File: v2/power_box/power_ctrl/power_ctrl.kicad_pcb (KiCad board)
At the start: 2 copper layers, 37 parts, among them J1 Atmega328, Q1 BC547, Q2 Q_PMOS_GDS, U1 7805

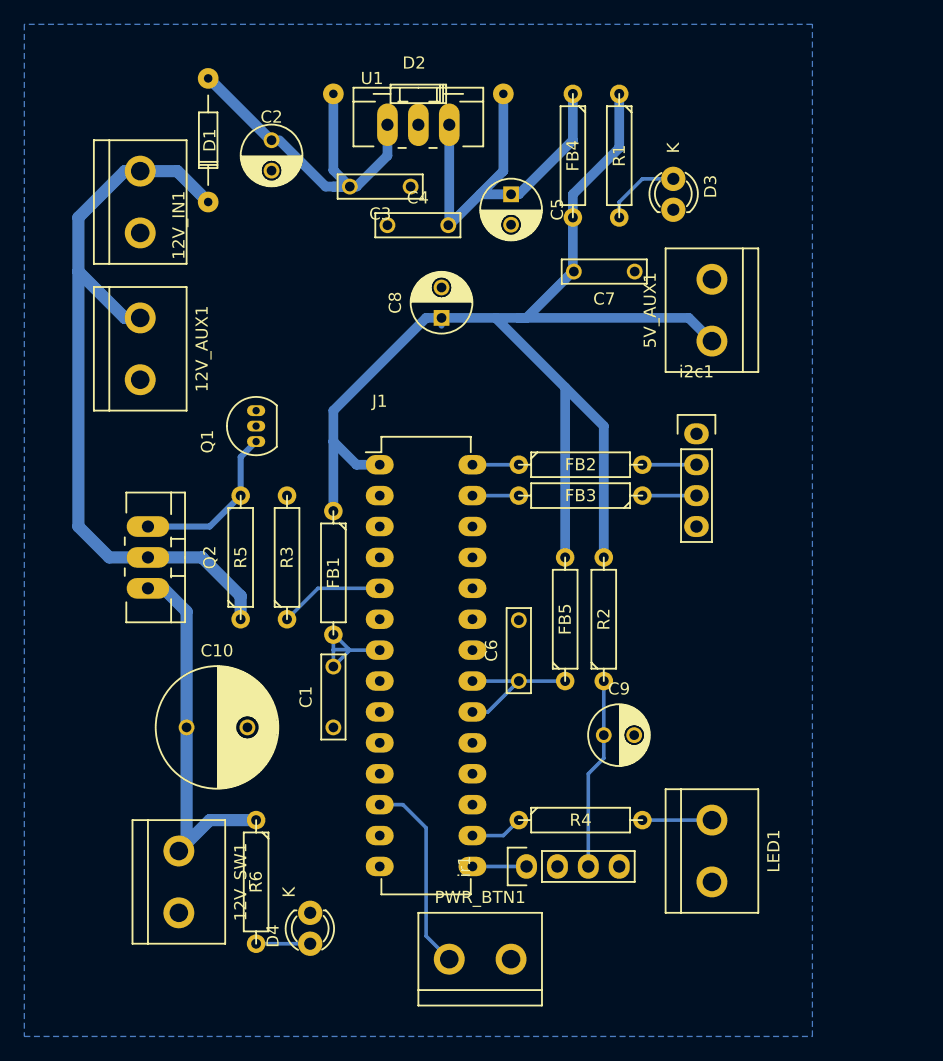
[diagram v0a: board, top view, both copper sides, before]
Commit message: update
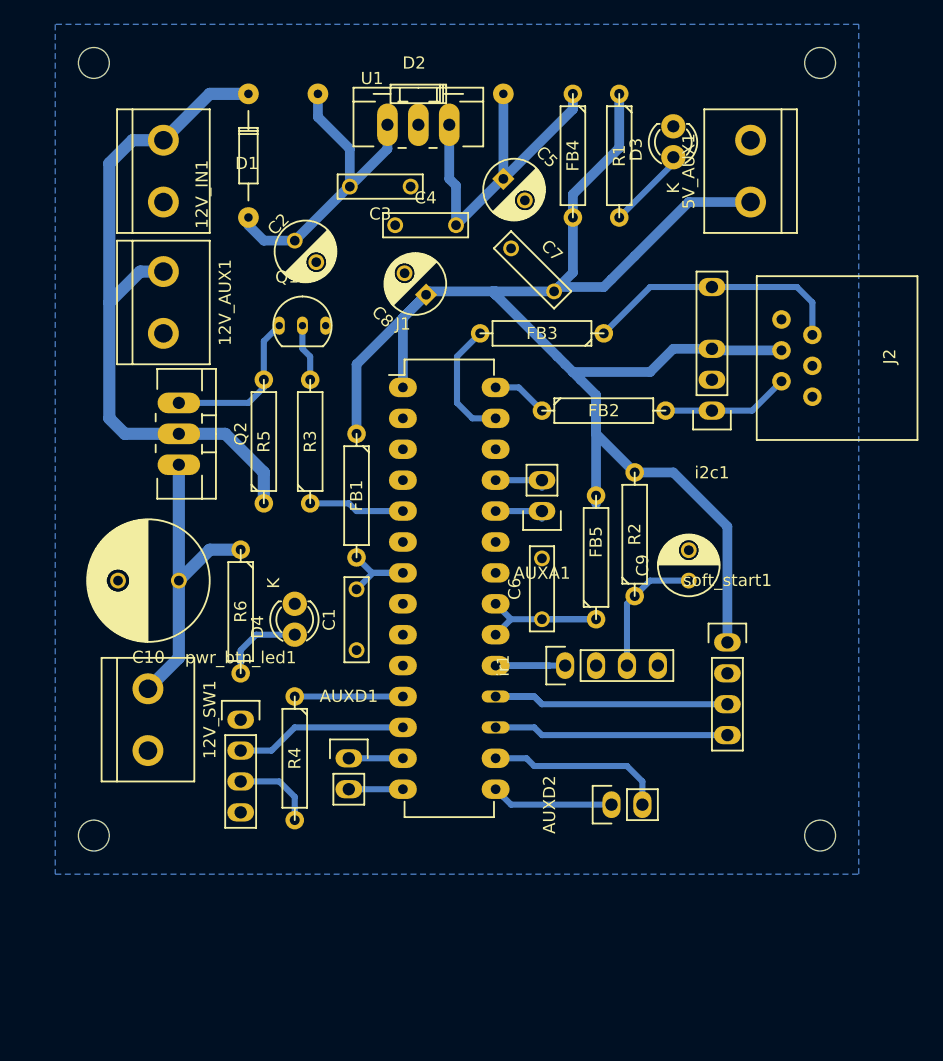
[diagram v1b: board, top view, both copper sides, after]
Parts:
- removed LED1, PWR_BTN1: CONN_2, Connect:bornier2
- added AUXA1: CONN_2, Pin_Headers:Pin_Header_Straight_1x02, F.Cu at (217.8, 94.6)
- added AUXD1: CONN_2, Pin_Headers:Pin_Header_Straight_1x02, F.Cu at (201.9, 114.9)
- added AUXD2: CONN_2, Pin_Headers:Pin_Header_Straight_1x02, F.Cu at (223.5, 118.7)
- added J2: RJ12, Connect:RJ12_E, F.Cu at (246.4, 81.9)
- added pwr_btn_led1: CONN_4, Pin_Headers:Pin_Header_Straight_1x04, F.Cu at (193.0, 111.8)
- added soft_start1: CONN_4, Pin_Headers:Pin_Header_Straight_1x04, F.Cu at (233.0, 105.4)
- i2c1: value CONN_4 -> CONN_01X05; footprint Pin_Headers:Pin_Header_Straight_1x04 -> Pin_Headers:Pin_Header_Straight_1x05
- moved D4 25.4 mm to (197.5, 102.2)
- moved R4 24.0 mm to (197.5, 114.9), turned to 270 degrees
- moved R6 22.3 mm to (193.0, 102.9)
- moved ir1 16.8 mm to (219.7, 107.3)
- moved C9 14.5 mm to (229.9, 100.3), turned to 90 degrees
- moved FB3 13.7 mm to (217.8, 80.0)
- moved 12V_SW1 13.6 mm to (185.4, 111.8)
- moved C10 12.1 mm to (188.0, 100.3), turned to 180 degrees
- moved 5V_AUX1 11.9 mm to (234.9, 66.7)
- moved Q2 10.5 mm to (188.0, 88.3)
- moved C7 10.3 mm to (215.3, 73.0), turned to 315 degrees
- moved Q1 9.86 mm to (196.8, 79.4), turned to 0 degrees
- moved R3 9.71 mm to (198.8, 88.9)
- moved R5 9.71 mm to (194.9, 88.9)
- moved D1 9.48 mm to (193.7, 60.3), turned to 270 degrees
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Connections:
- J1 pad 11: (no net) -> /PWR_LED
- J1 pad 13: (no net) -> /AUXD1
- J1 pad 14: (no net) -> /AUXD2
- J1 pad 15: /IR_IN -> /AUXD3
- J1 pad 16: /PWR_LED -> /AUXD4
- J1 pad 17: (no net) -> /EN_R2
- J1 pad 18: (no net) -> /EN_R1
- J1 pad 19: (no net) -> /IR_IN
- J1 pad 24: (no net) -> /AUXA1
- J1 pad 25: (no net) -> /AUXA2
- i2c1 pad 1: GND -> /SCL
- i2c1 pad 2: /SCL -> GND
- i2c1 pad 3: /SDA -> /5V
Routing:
- net /EN_R1: track 0.00 -> 23.4 mm
- net /5V: track 115.3 -> 136.9 mm
- net /EN_R2: track 0.00 -> 19.3 mm
- net /SDA: track 4.44 -> 21.9 mm
- net /AUXD4: track 0.00 -> 14.8 mm
- net Net-(C2-Pad1): track 39.6 -> 27.8 mm
- net /AUXD3: track 0.00 -> 10.9 mm
- net /12V_SW: track 32.2 -> 25.6 mm
- net Net-(FB3-Pad2): track 3.81 -> 10.2 mm
- net /SCL: track 4.44 -> 10.5 mm
- net /IR_IN: track 4.44 -> 10.2 mm
- net Net-(C9-Pad1): track 15.8 -> 10.9 mm
- net Net-(Q1-Pad2): track 0.00 -> 4.71 mm
- net /PWR_LED: track 4.34 -> 8.89 mm
- net /AUXD2: track 0.00 -> 4.44 mm
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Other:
- board outline added: 62.2 x 66 mm
